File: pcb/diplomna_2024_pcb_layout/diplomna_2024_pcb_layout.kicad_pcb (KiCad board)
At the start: 4 copper layers, 95 x 95 mm, 15 parts

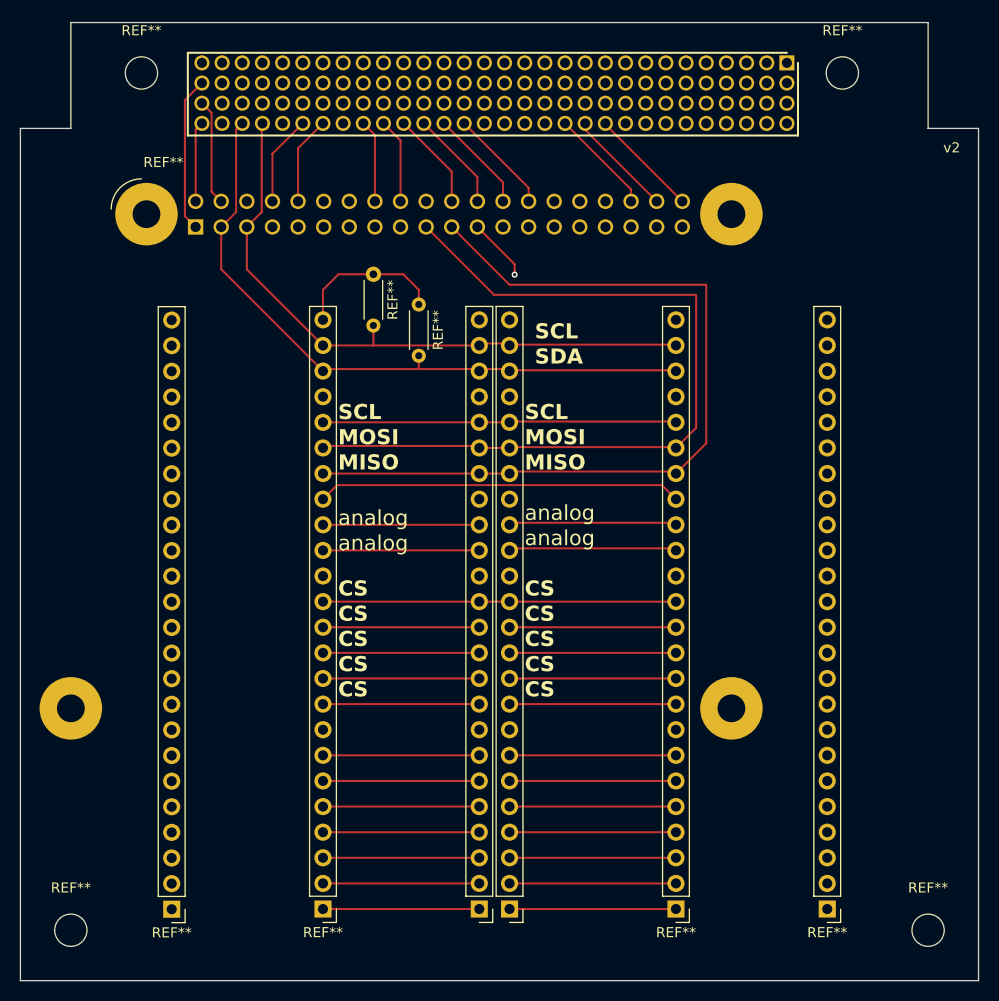
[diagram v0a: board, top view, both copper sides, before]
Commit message: pcb chnge
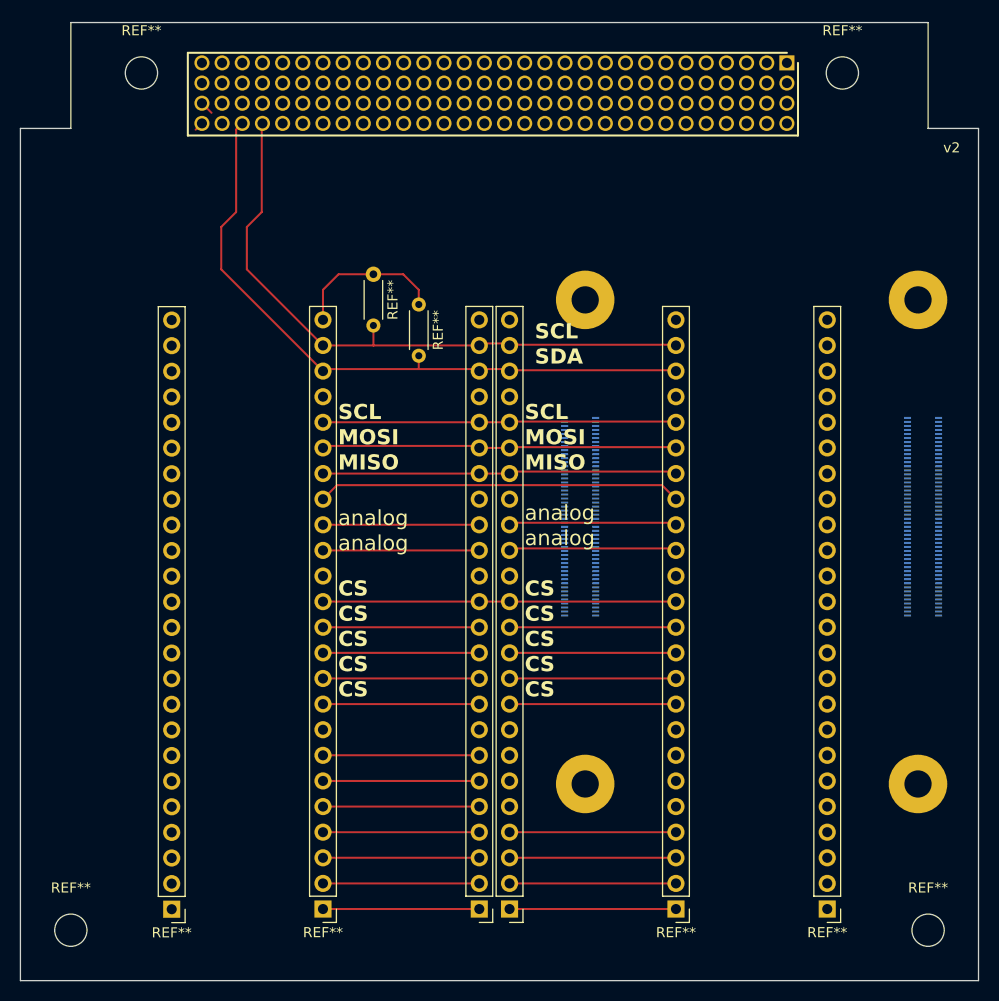
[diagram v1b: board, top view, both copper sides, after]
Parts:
- removed ?: , 
- removed the REF** at (207.5, 94.0)
- added REF**: MODULE_CM4102008, rp1:MODULE_CM4102008, B.Cu at (228.5, 102.0)
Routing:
- net I/O: track 312.8 -> 175.2 mm
- net miso: track 82.7 -> 35.1 mm
- net mosi: track 80.7 -> 35.1 mm
- net scl: track 77.6 -> 35.7 mm, vias 1 -> 0
- net VDD: track 123.3 -> 107.0 mm
- net 3.3v: track 15.4 -> 0.00 mm
- net tx: track 8.98 -> 0.00 mm
- net rx: track 8.75 -> 0.00 mm

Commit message: testing and presentation changes
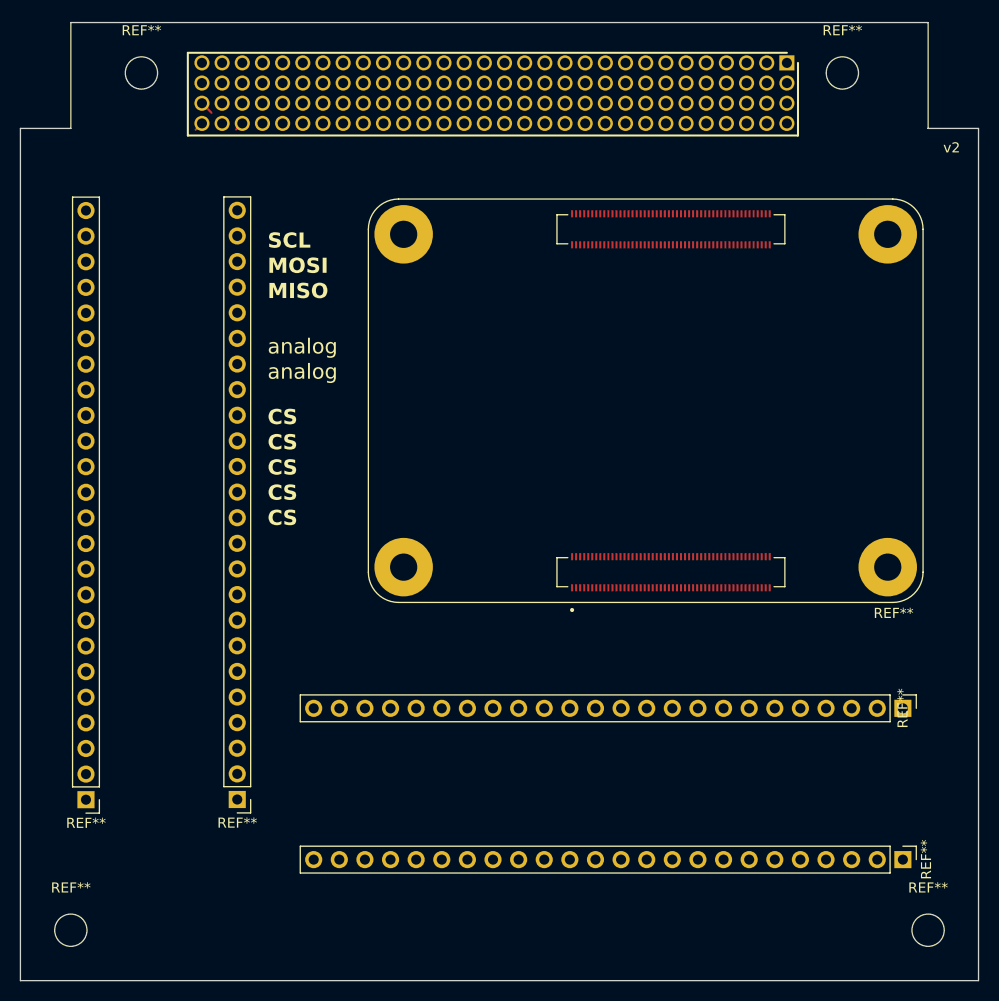
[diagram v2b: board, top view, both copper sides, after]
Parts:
- removed the REF** at (191.0, 75.5)
- removed the REF** at (195.5, 78.5)
- removed the REF** at (204.5, 138.4)
- removed the REF** at (201.5, 138.4)
- REF**: moved to F.Cu
- moved REF** 23.0 mm to (243.5, 133.5), turned to -90 degrees
- moved REF** 21.3 mm to (243.5, 118.5), turned to -90 degrees
- moved REF** 17.5 mm to (218.0, 88.0), turned to 180 degrees
- moved REF** 13.8 mm to (177.5, 127.5)
- moved REF** 13.8 mm to (162.5, 127.6)
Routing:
- net CS: track 199.3 -> 0.00 mm
- net I/O: track 175.2 -> 0.74 mm
- net VDD: track 107.0 -> 2.23 mm
- net sda_i2c: track 66.5 -> 0.87 mm
- net analog: track 64.3 -> 0.00 mm
- net scl_i2c: track 63.4 -> 0.10 mm
- net scl: track 35.7 -> 0.00 mm
- net miso: track 35.1 -> 0.00 mm
- net mosi: track 35.1 -> 0.00 mm
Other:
- board text removed: "SDA"
